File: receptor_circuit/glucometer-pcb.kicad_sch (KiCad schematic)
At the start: 17 parts, among them IC1 RC4558IP, IC2 LM1458N, IC3 RC4558IP

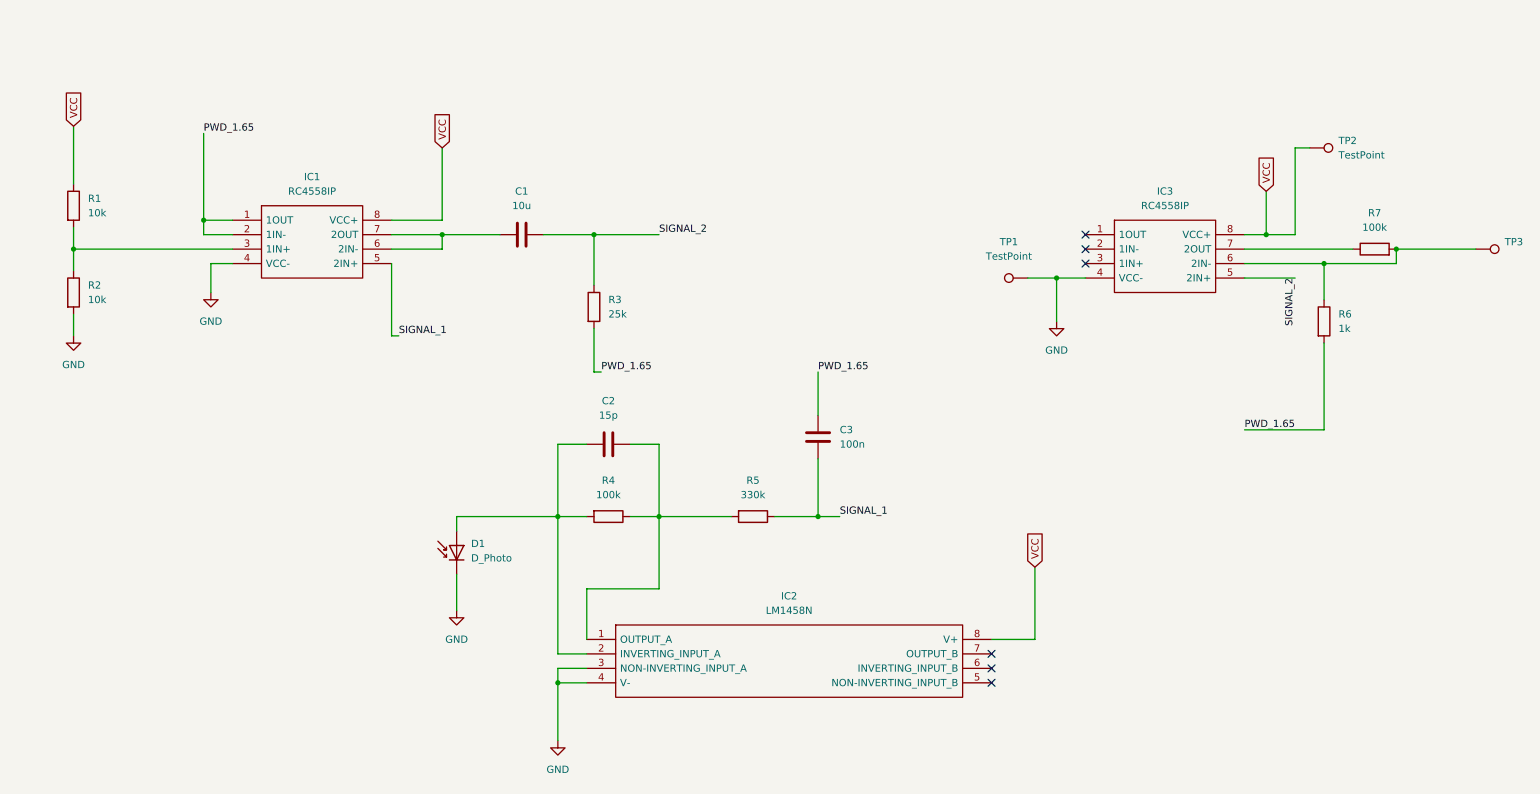
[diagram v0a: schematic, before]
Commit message: fixed PCB
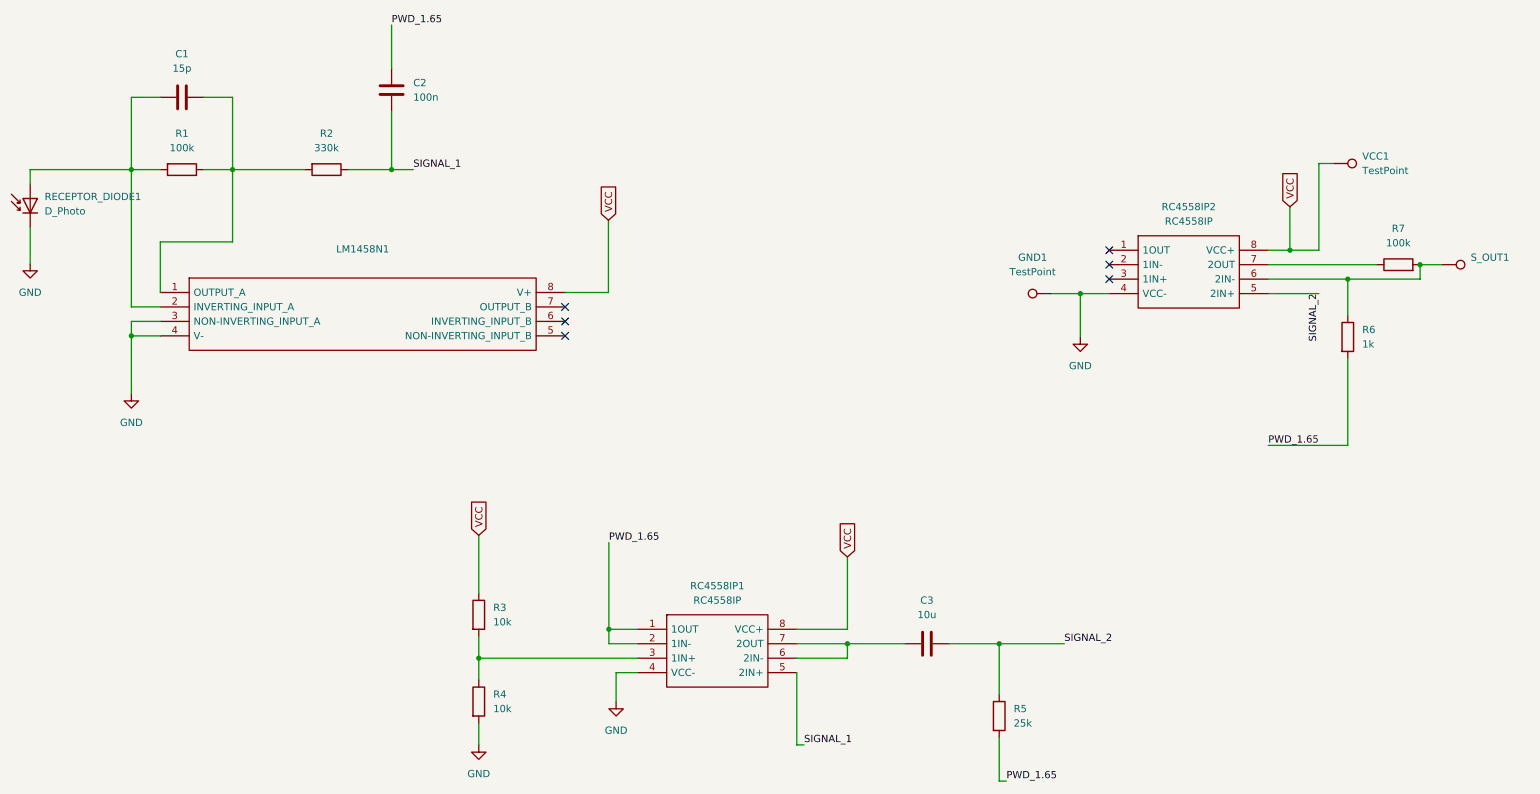
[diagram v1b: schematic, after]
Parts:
- LM1458N1: renamed from IC2; value LM1458N -> (none)
- S_OUT1: renamed from TP3; footprint TestPoint:TestPoint_Keystone_5015_Micro-Minature -> (none)
- renumbered C2 to C1, C3 to C2, C1 to C3, TP1 to GND1, R4 to R1, R5 to R2, R1 to R3, R2 to R4, R3 to R5, IC1 to RC4558IP1, IC3 to RC4558IP2, D1 to RECEPTOR_DIODE1, TP2 to VCC1
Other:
- moved on the sheet: C1, C2, C3, GND1, LM1458N1, R1, R2, R3, R4, R5, R6, R7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
